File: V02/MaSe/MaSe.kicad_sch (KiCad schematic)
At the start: 44 parts, among them J1 Conn_02x08_Odd_Even, J2 ALIM_BAT, J3 Conn_02x08_Odd_Even, J4 Conn_01x02, Q2 BSS83P, Q3 BSS83P, SW1 Push_Button, SW10 Push_Button, SW2 Push_Button, SW3 RotaryEncoder, SW4 Push_Button, SW5 Push_Button, SW6 Push_Button, SW7 Push_Button, SW8 Push_Button, SW9 Push_Button, U1 TCR2EF19, U2 PMW3360, U3 TLV73333PDBV, U4 AP130-33SA, U5 ESP32-S3-DevKitC, U6 AP130-33SA, U8 NRF24L01_Breakout

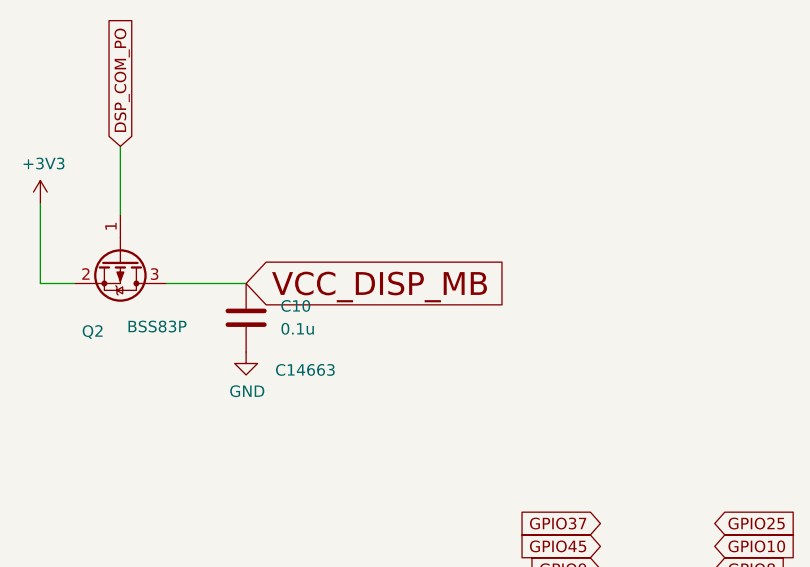
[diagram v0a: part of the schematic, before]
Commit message: e
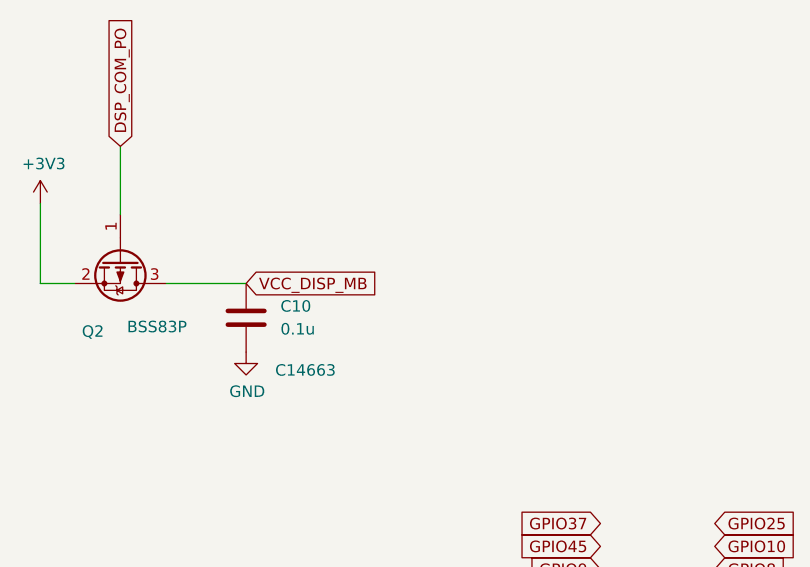
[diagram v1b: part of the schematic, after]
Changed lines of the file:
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@@
 		(effects
 			(font
-				(size 2.54 2.54)
+				(size 1.27 1.27)
 			)
 			(justify left)
 		)
 		(property "Intersheetrefs" "${INTERSHEET_REFS}"
-			(at 139.1601 -33.02 0)
+			(at 124.1905 -33.02 0)
 			(effects
 				(font
